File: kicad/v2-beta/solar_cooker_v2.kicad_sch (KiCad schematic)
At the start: 17 parts, among them J1 M20-9980346, J2 Conn_01x06_Pin, J3 Conn_01x14_Pin, J4 M20-9980346, J5 MUSB-05-X-B-SM-A, SW2 SW_Push_Dual, U1 ATmega328P-P, U2 ATmega16U2-A, U3 LP2985-3.3, Y1 Resonator

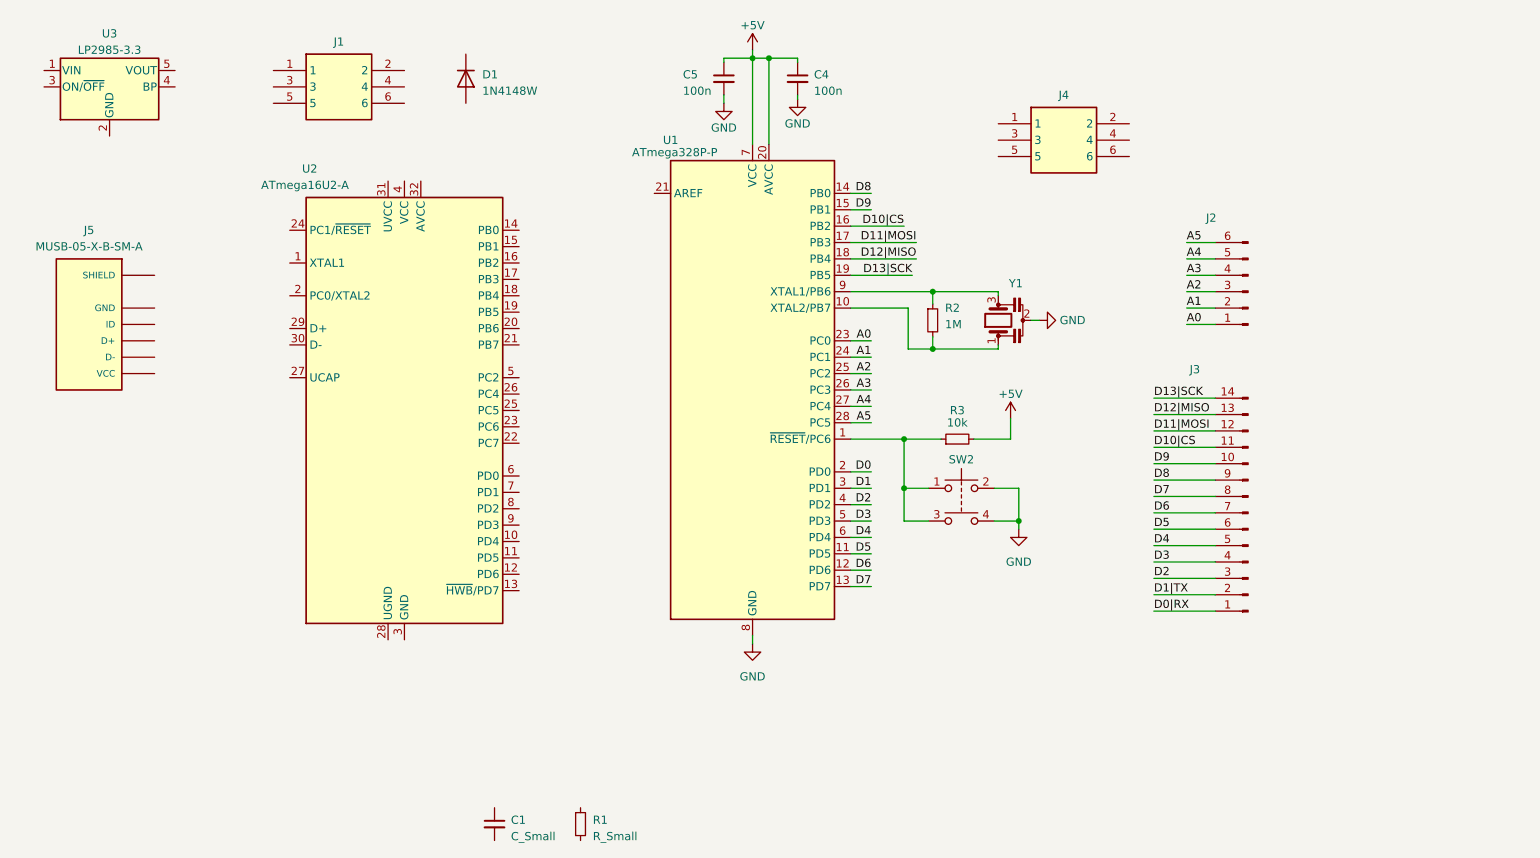
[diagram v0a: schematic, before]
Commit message: kicad update
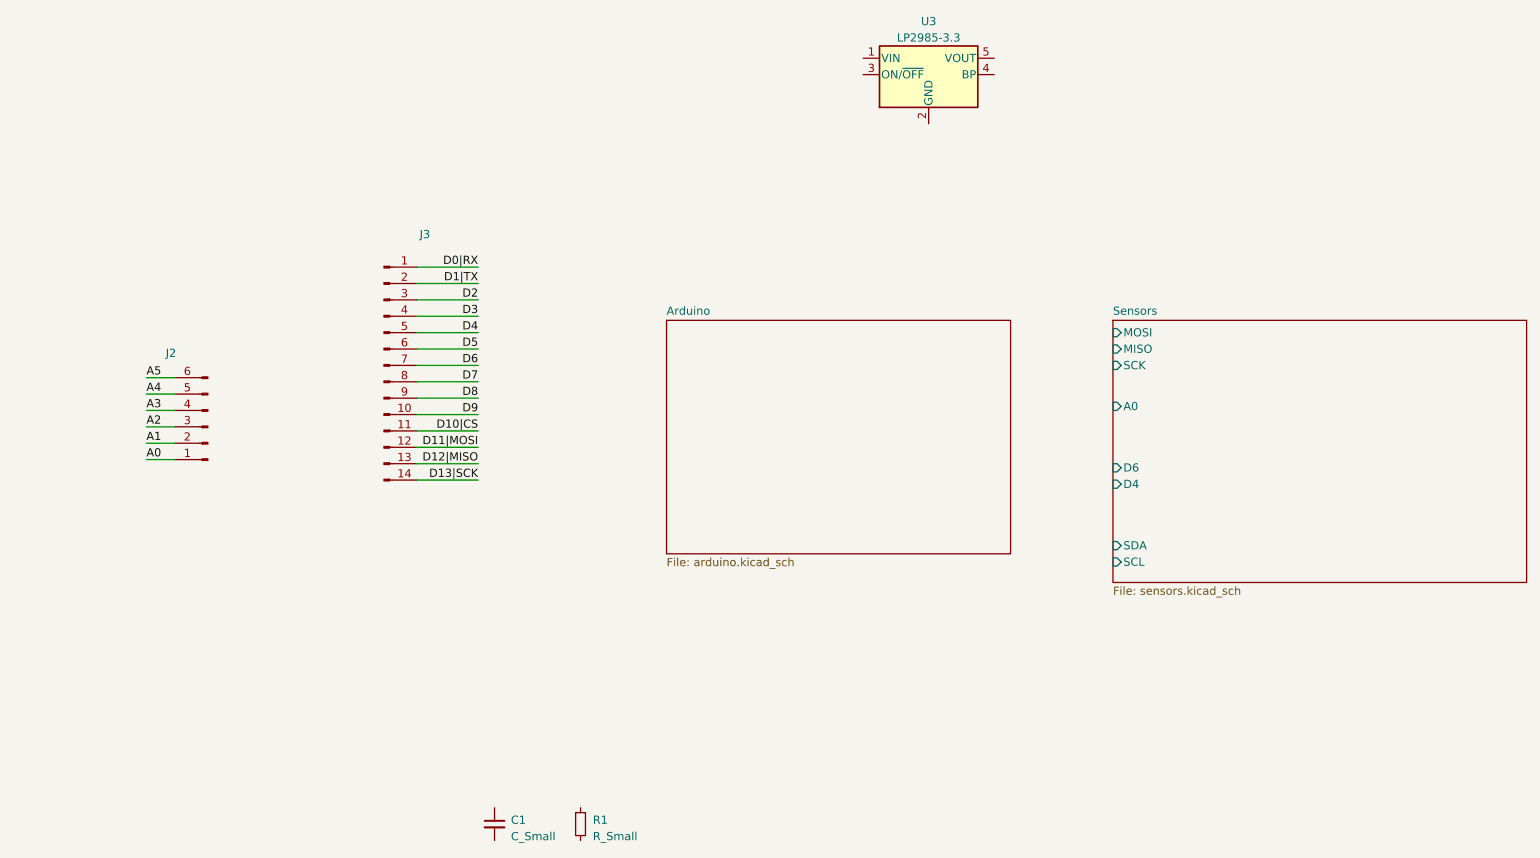
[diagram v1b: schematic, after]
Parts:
- removed C4, C5: 100n, Capacitor_SMD:C_01005_0402Metric, symbol Device:C_Small
- removed D1: 1N4148W, Diode_SMD:D_SOD-123, symbol Diode:1N4148W
- removed J1, J4: M20-9980346, HDRV6W64P254_2X3_762X508X868P, symbol M20-9980346:M20-9980346
- removed J5: MUSB-05-X-B-SM-A, SAMTEC_MUSB-05-X-B-SM-A, symbol MUSB-05-X-B-SM-A:MUSB-05-X-B-SM-A
- removed R2: 1M, Resistor_SMD:R_01005_0402Metric, symbol Device:R_Small
- removed R3: 10k, Resistor_SMD:R_01005_0402Metric, symbol Device:R_Small
- removed SW2: SW_Push_Dual, push button:SMT3-01-Z, symbol Switch:SW_Push_Dual
- removed U1: ATmega328P-P, Package_DIP:DIP-28_W7.62mm, symbol MCU_Microchip_ATmega:ATmega328P-P
- removed U2: ATmega16U2-A, Package_QFP:TQFP-32_7x7mm_P0.8mm, symbol MCU_Microchip_ATmega:ATmega16U2-A
- removed Y1: Resonator, resonator:OSC_CSTCE16M0V53-R0, symbol Device:Resonator
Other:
- added sheet Arduino (arduino.kicad_sch)
- added sheet Sensors (sensors.kicad_sch)
- moved on the sheet: J2, J3, U3
